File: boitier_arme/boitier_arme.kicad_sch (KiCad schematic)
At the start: 8 parts, among them J1 Conn_01x02_Pin, J2 Battery, U1 XIAO-nRF52840-SMD

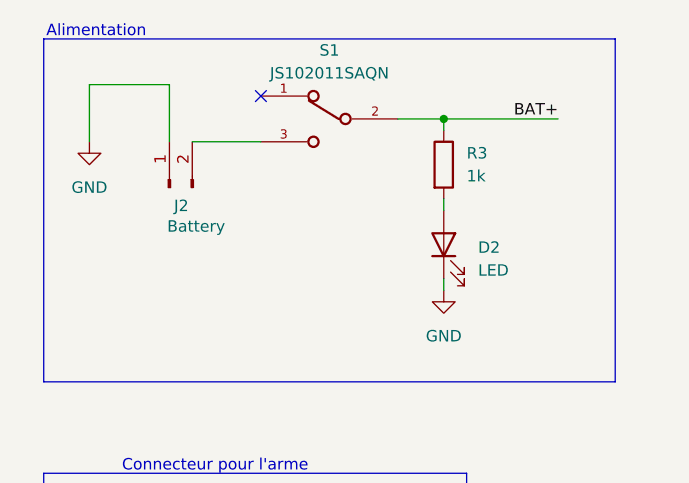
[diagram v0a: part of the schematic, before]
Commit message: a jour
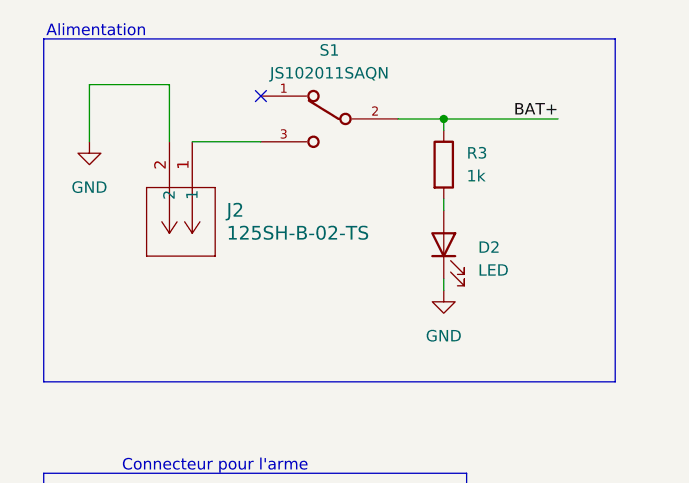
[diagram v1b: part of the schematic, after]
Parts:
- removed J2: Battery, Connector_JST:JST_XH_B2B-XH-A_1x02_P2.50mm_Vertical, symbol Connector:Conn_01x02_Pin
- added J2: 125SH-B-02-TS, CONN_125SH-B-02-TS_ADM, symbol 2025-07-15_01-55-54:125SH-B-02-TS
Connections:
- net GND: now also J2.2
- net at S1.3: now also J2.1
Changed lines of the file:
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@@
+	)
+	(symbol
+		(lib_id "2025-07-15_01-55-54:125SH-B-02-TS")
+		(at 30.48 27.94 270)
+		(unit 1)
+		(exclude_from_sim no)
+		(in_bom yes)
+		(on_board yes)
+		(dnp no)
+		(fields_autoplaced yes)
+		(property "Reference" "J2"
+			(at 34.29 35.5599 90)
+			(effects
+				(font
+					(size 1.524 1.524)
+				)
+				(justify left)
+			)
+		)
+		(property "Value" "125SH-B-02-TS"
+			(at 34.29 38.0999 90)
+			(effects
+				(font
+					(size 1.524 1.524)
+				)
+				(justify left)
+			)
+		)
+		(property "Footprint" "CONN_125SH-B-02-TS_ADM"
+			(at 30.48 27.94 0)
+			(effects
+				(font
+					(size 1.27 1.27)
+					(italic yes)
+				)
+				(hide yes)
+			)
+		)
+		(property "Datasheet" "125SH-B-02-TS"
+			(at 30.48 27.94 0)
+			(effects
+				(font
+					(size 1.27 1.27)
+					(italic yes)
+				)
+				(hide yes)
+			)
+		)
+		(property "Description" ""
+			(at 30.48 27.94 0)
+			(effects
+				(font
+					(size 1.27 1.27)
+				)
+				(hide yes)
+			)
+		)
+		(pin "1"
+		)
+		(pin "2"
+		)
+		(instances
+			(project ""
+				(path "/98d1fd79-24f6-41e8-83f3-a60accf8c857"
+					(reference "J2")
+					(unit 1)
+				)
+			)
+		)
 	)
 	(symbol
@@
 					(unit 1)
 				)
-			)
-		)
-	)
-	(symbol
-		(lib_id "Connector:Conn_01x02_Pin")
-		(at 27.94 33.02 90)
-		(unit 1)
-		(exclude_from_sim no)
-		(in_bom yes)
-		(on_board yes)
-		(dnp no)
-		(property "Reference" "J2"
-			(at 28.448 35.052 90)
-			(effects
-				(font
-					(size 1.27 1.27)
-				)
-				(justify right)
-			)
-		)
-		(property "Value" "Battery"
-			(at 27.686 37.338 90)
-			(effects
-				(font
-					(size 1.27 1.27)
-				)
-				(justify right)
-			)
-		)
-		(property "Footprint" "Connector_JST:JST_XH_B2B-XH-A_1x02_P2.50mm_Vertical"
-			(at 27.94 33.02 0)
-			(effects
-				(font
-					(size 1.27 1.27)
-				)
-				(hide yes)
-			)
-		)
-		(property "Datasheet" "~"
-			(at 27.94 33.02 0)
-			(effects
-				(font
-					(size 1.27 1.27)
-				)
-				(hide yes)
-			)
-		)
-		(property "Description" "Generic connector, single row, 01x02, script generated"
-			(at 27.94 33.02 0)
-			(effects
-				(font
-					(size 1.27 1.27)
-				)
-				(hide yes)
-			)
-		)
-		(pin "1"
-		)
-		(pin "2"
-		)
-		(instances
-			(project "boitier_arme"
-				(path "/98d1fd79-24f6-41e8-83f3-a60accf8c857"
-					(reference "J2")
-					(unit 1)
-				)

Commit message: a jour
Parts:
- J1: footprint Connector_JST:JST_XH_B2B-XH-A_1x02_P2.50mm_Vertical -> Connector_JST:JST_XH_S2B-XH-A-1_1x02_P2.50mm_Horizontal
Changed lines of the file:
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@@
 			)
 		)
-		(property "Footprint" "Connector_JST:JST_XH_B2B-XH-A_1x02_P2.50mm_Vertical"
+		(property "Footprint" "Connector_JST:JST_XH_S2B-XH-A-1_1x02_P2.50mm_Horizontal"
 			(at 41.91 78.74 0)
 			(effects
